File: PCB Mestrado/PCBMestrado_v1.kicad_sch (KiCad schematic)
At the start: 32 parts, among them J2 USB_C_Receptacle_USB2.0, SW1 SW_Push_Dual, SW2 SW_Push_Dual, U2 STM32F446RETx, U6 TJA1042T-3, Y1 8MHz

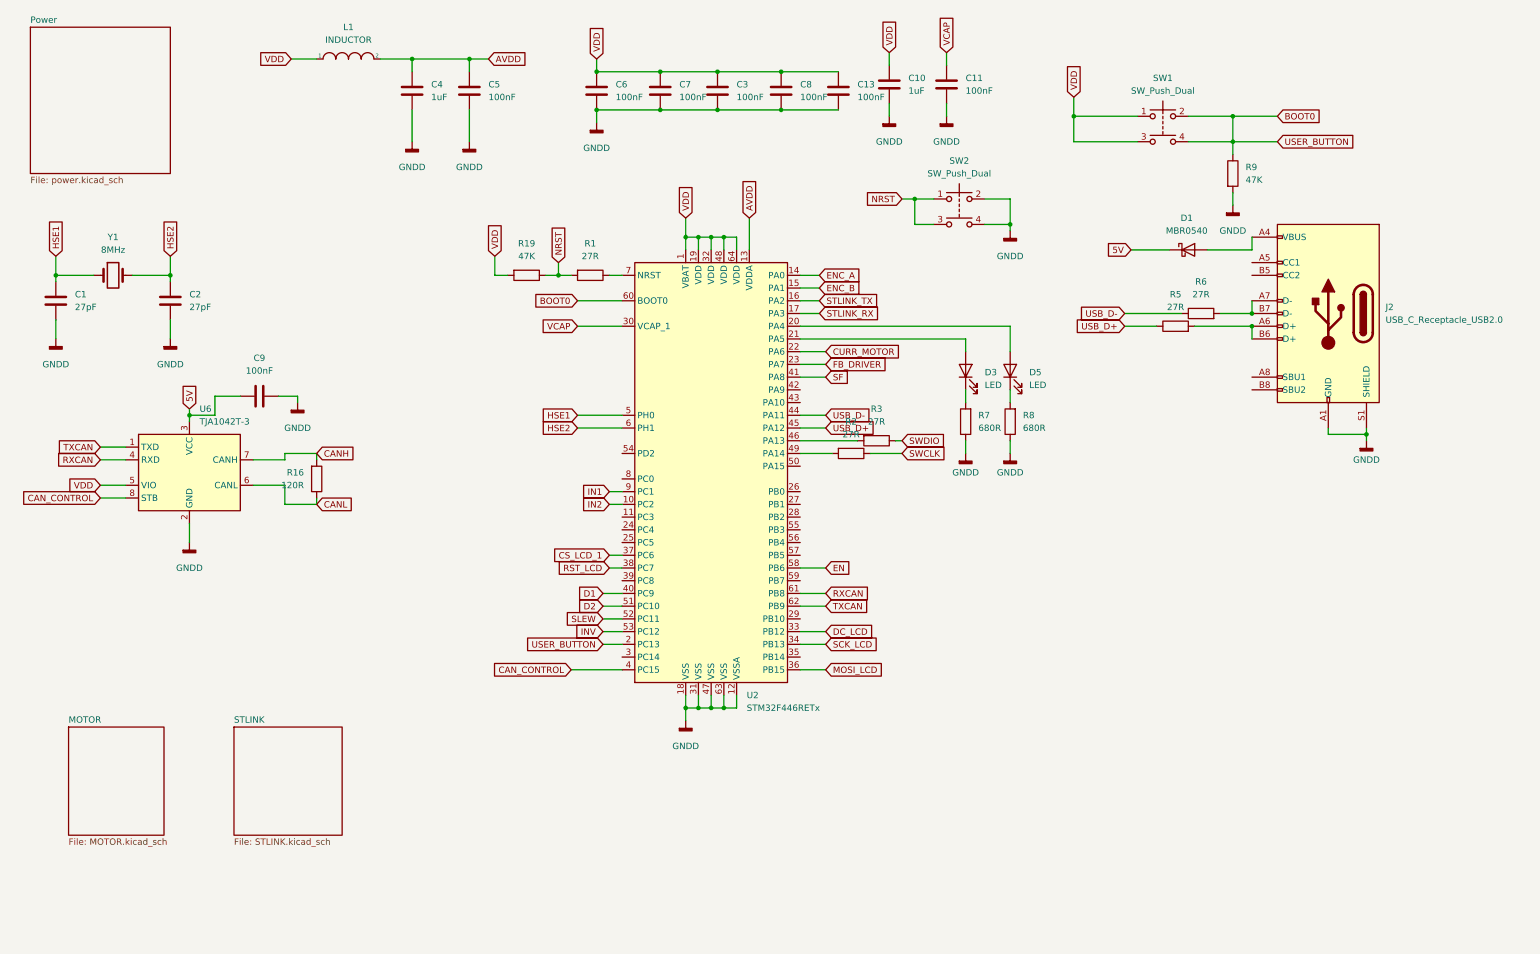
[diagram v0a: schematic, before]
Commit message: BUILDING
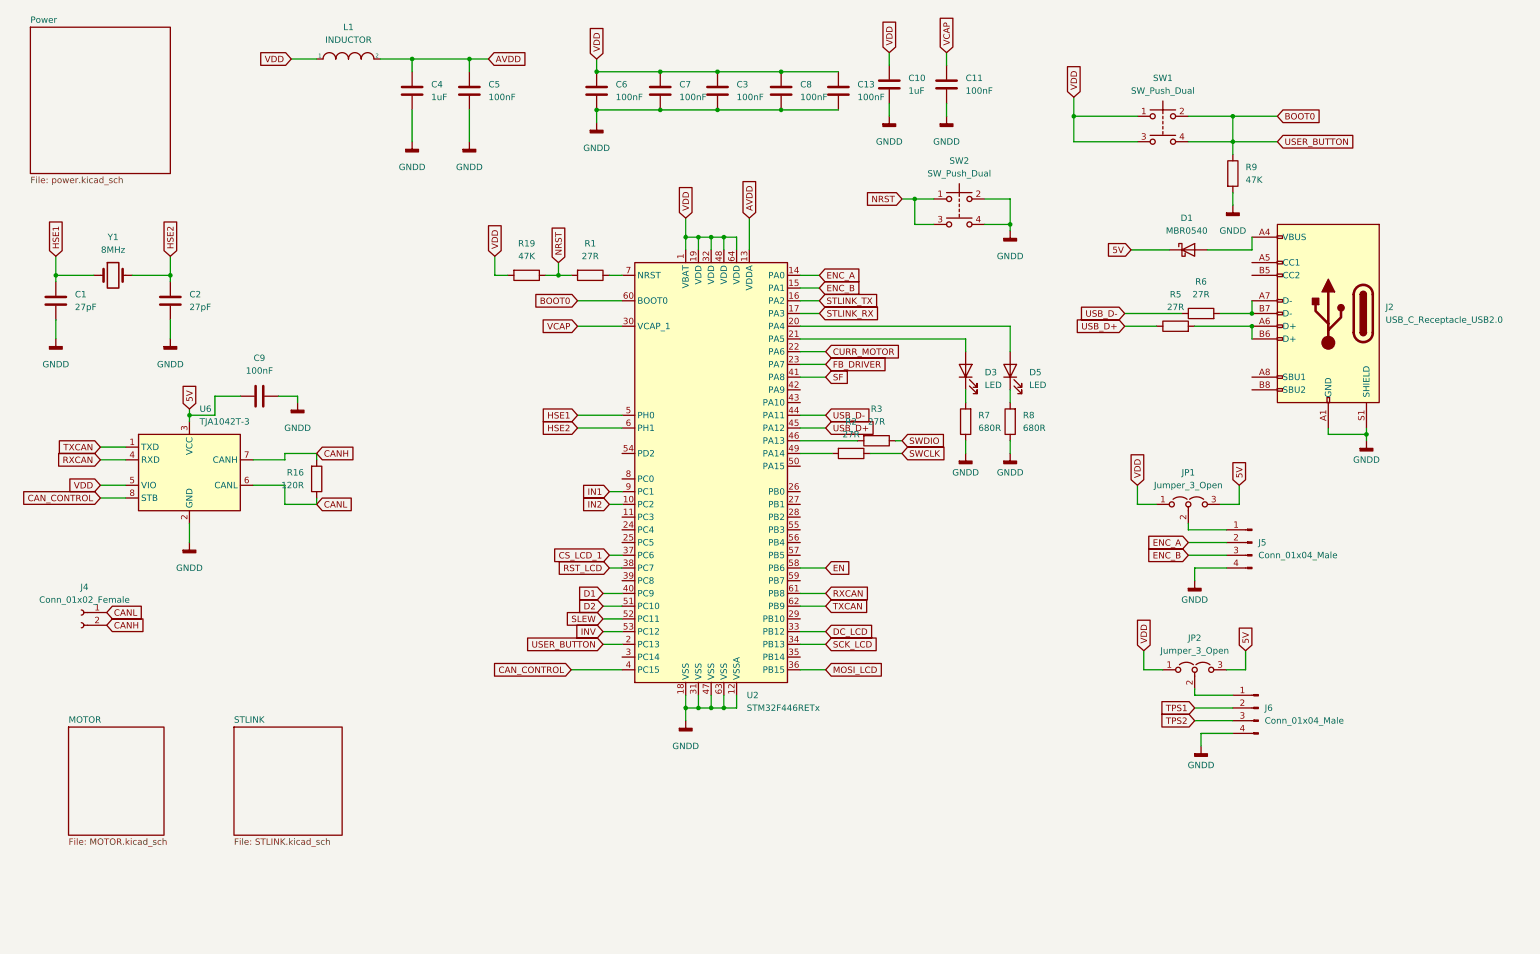
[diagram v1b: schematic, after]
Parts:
- added J4: Conn_01x02_Female, Connector_Phoenix_MSTB:PhoenixContact_MSTBA_2,5_2-G-5,08_1x02_P5.08mm_Horizontal, symbol Connector:Conn_01x02_Female
- added J5, J6: Conn_01x04_Male, Connector_JST:JST_EH_B4B-EH-A_1x04_P2.50mm_Vertical, symbol Connector:Conn_01x04_Male
- added JP1, JP2: Jumper_3_Open, Jumper:SolderJumper-3_P2.0mm_Open_TrianglePad1.0x1.5mm, symbol Jumper:Jumper_3_Open
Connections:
- net 5V: now also JP1.3 (B), JP2.3 (B)
- net CANH: now also J4.2 (Pin_2)
- net CANL: now also J4.1 (Pin_1)
- net ENC_A: now also J5.2 (Pin_2)
- net ENC_B: now also J5.3 (Pin_3)
- net GNDD: now also J5.4 (Pin_4), J6.4 (Pin_4)
- net VDD: now also JP1.1 (A), JP2.1 (A)
- new net: J6.1 (Pin_1), JP2.2 (C)
- new net: J5.1 (Pin_1), JP1.2 (C)
- new net TPS1: J6.2 (Pin_2)
- new net TPS2: J6.3 (Pin_3)

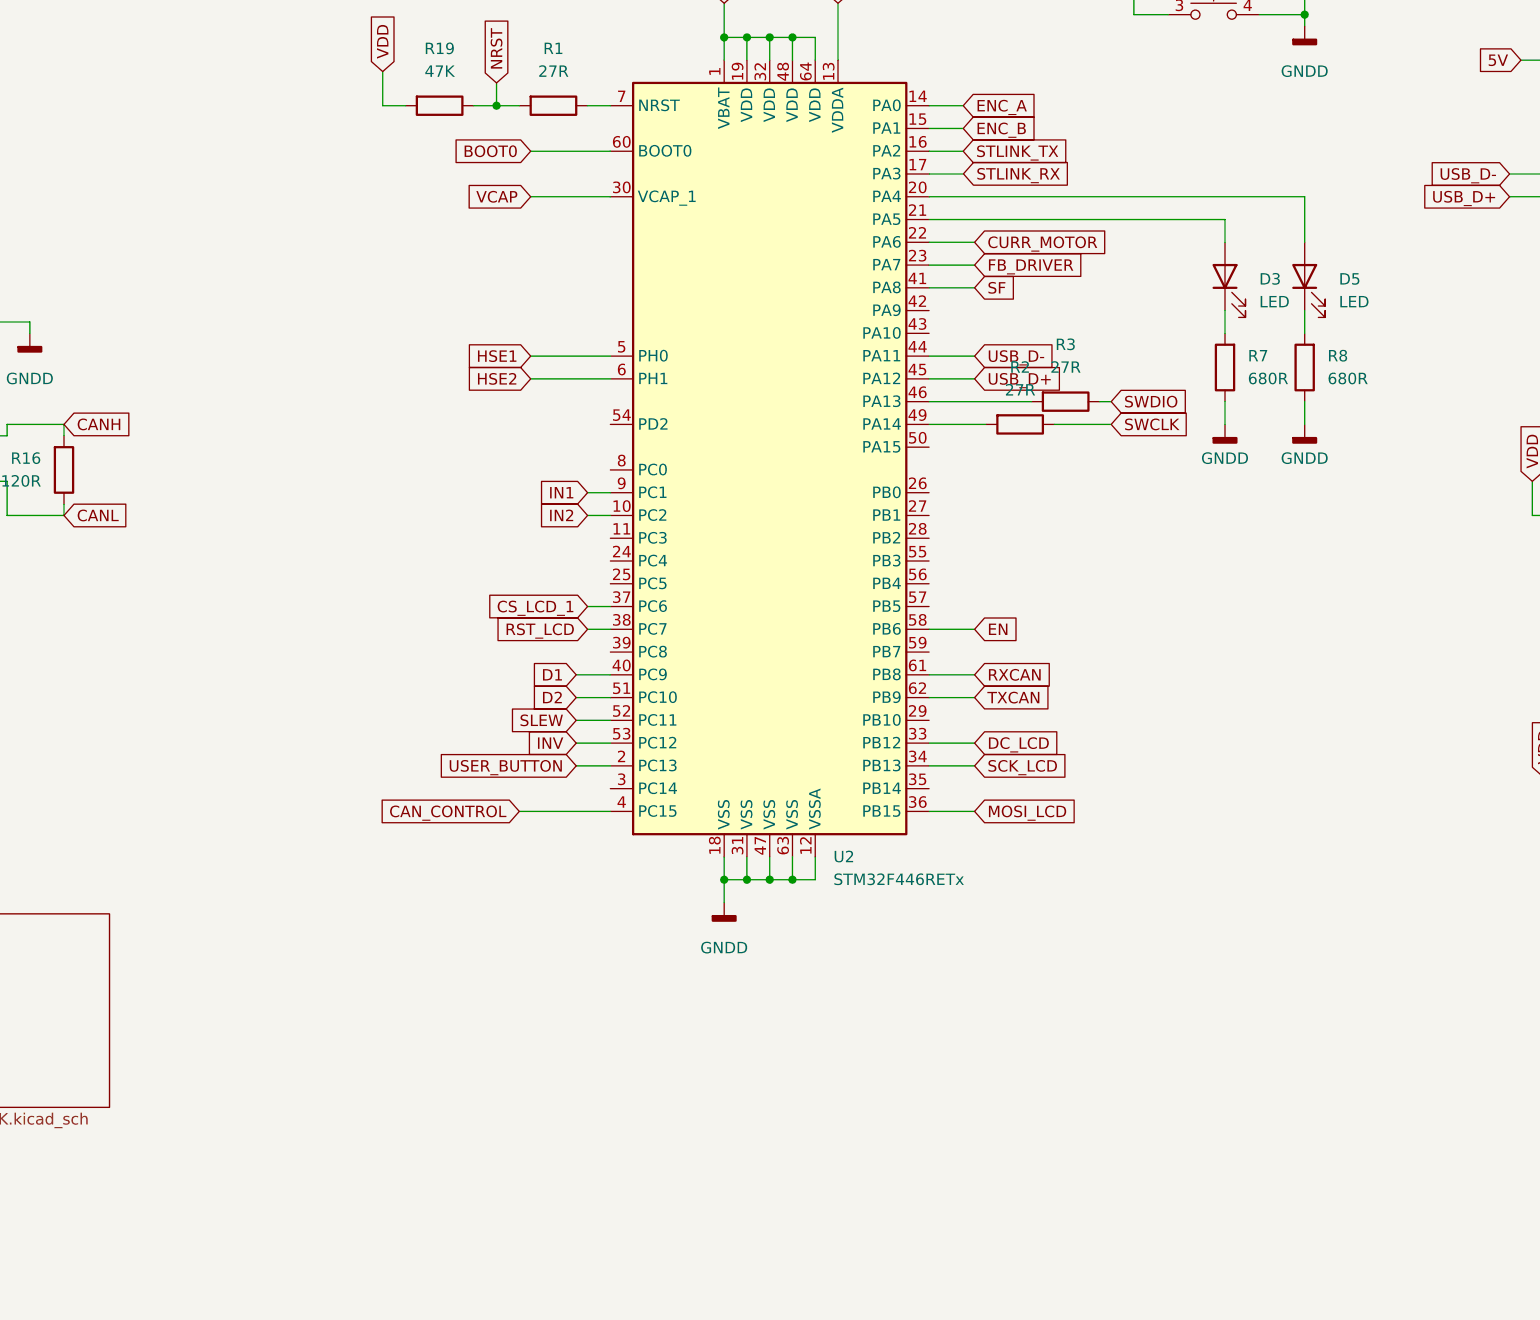
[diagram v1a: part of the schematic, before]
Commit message: build
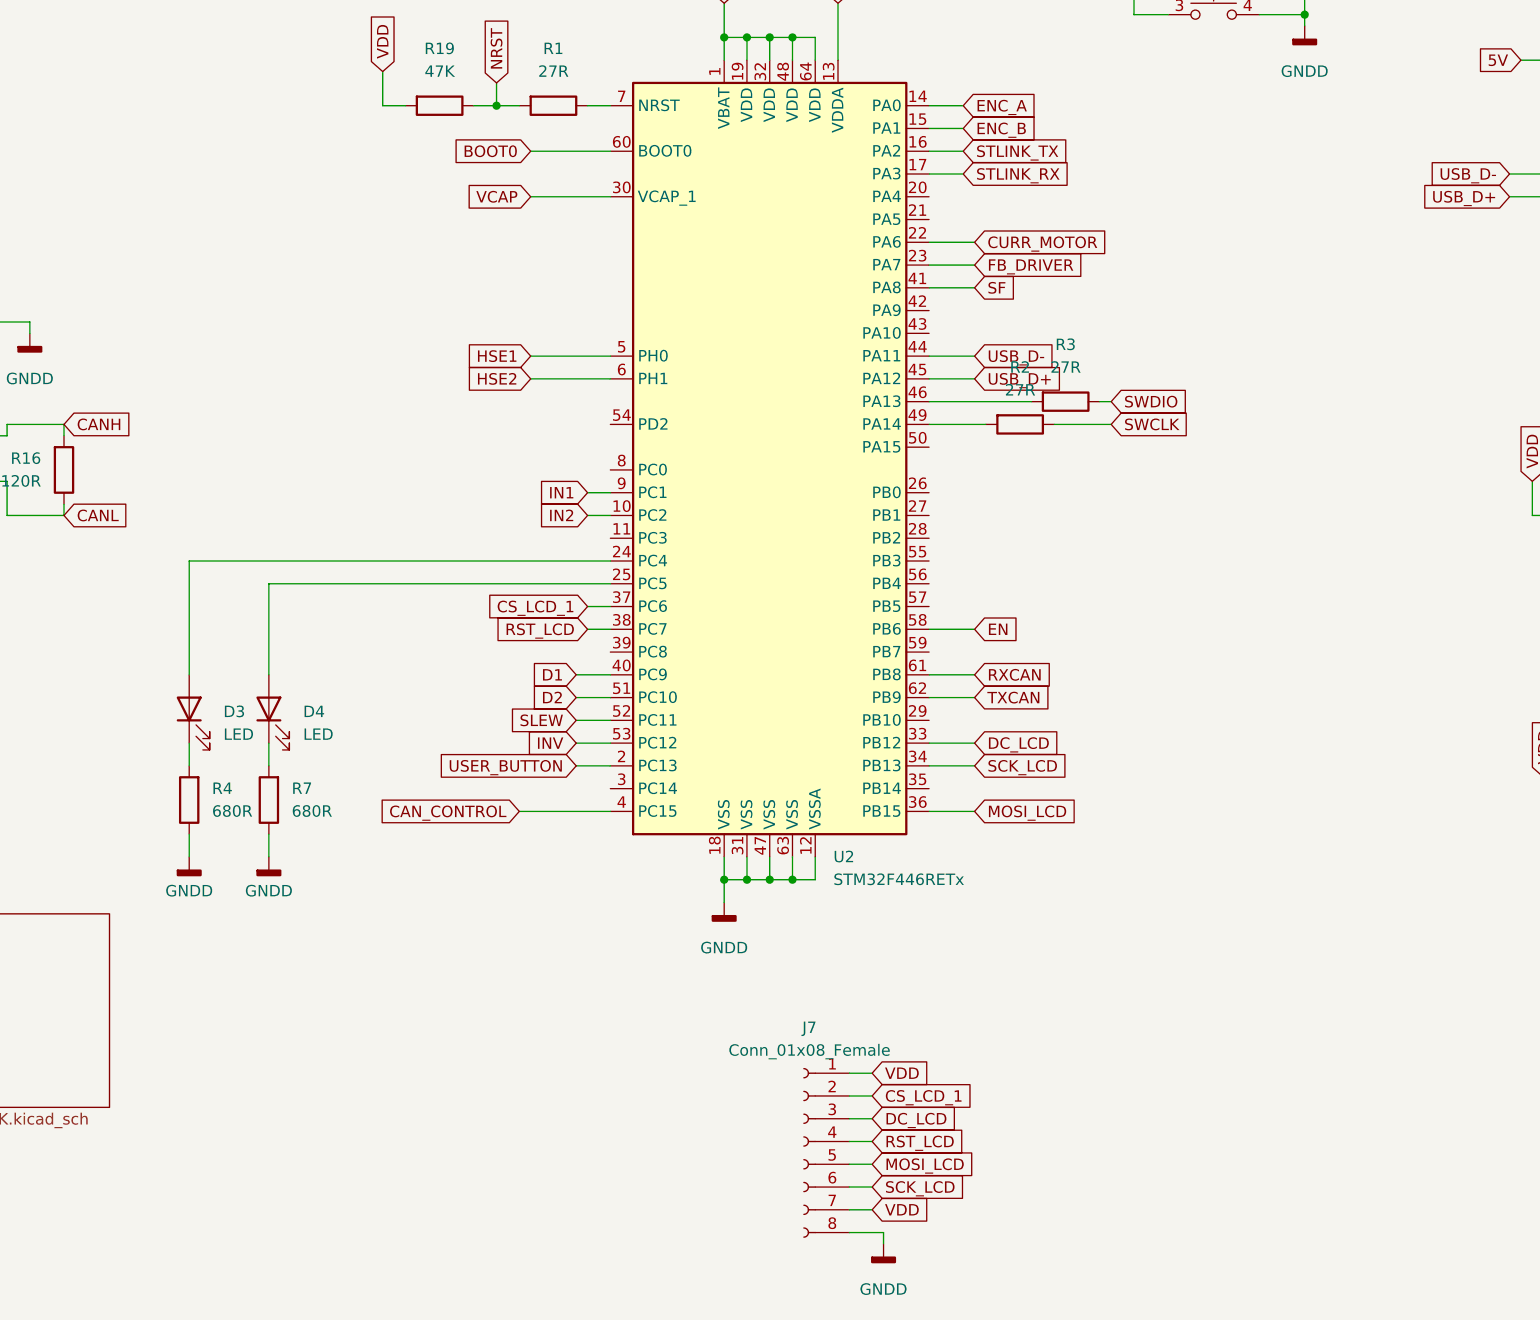
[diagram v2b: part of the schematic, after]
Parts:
- removed D5: LED, LED_SMD:LED_0603_1608Metric, symbol Device:LED
- removed R8: 680R, Resistor_SMD:R_0603_1608Metric, symbol Device:R
- added D4: LED, LED_SMD:LED_0603_1608Metric, symbol Device:LED
- added J7: Conn_01x08_Female, Connector_JST:JST_EH_B8B-EH-A_1x08_P2.50mm_Vertical, symbol Connector:Conn_01x08_Female
- added R4: 680R, Resistor_SMD:R_0603_1608Metric, symbol Device:R
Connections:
- net CS_LCD_1: now also J7.2 (Pin_2)
- net DC_LCD: now also J7.3 (Pin_3)
- net GNDD: now also J7.8 (Pin_8), R4.1
- net MOSI_LCD: now also J7.5 (Pin_5)
- net RST_LCD: now also J7.4 (Pin_4)
- net SCK_LCD: now also J7.6 (Pin_6)
- net STLINK_RX: now also U2.17 (PA3)
- net VDD: now also J7.1 (Pin_1), J7.7 (Pin_7)
- net at U2.21 (PA5): no longer D3.2 (A)
- net at U2.24 (PC4): now also D3.2 (A)
- net at U2.25 (PC5): now also D4.2 (A)
- net at R7.2: now also D4.1 (K); no longer D3.1 (K)
- new net: D3.1 (K), R4.2
